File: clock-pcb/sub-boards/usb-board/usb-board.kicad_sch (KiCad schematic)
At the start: 5 parts, among them J1 USB4140-GF-0070-C

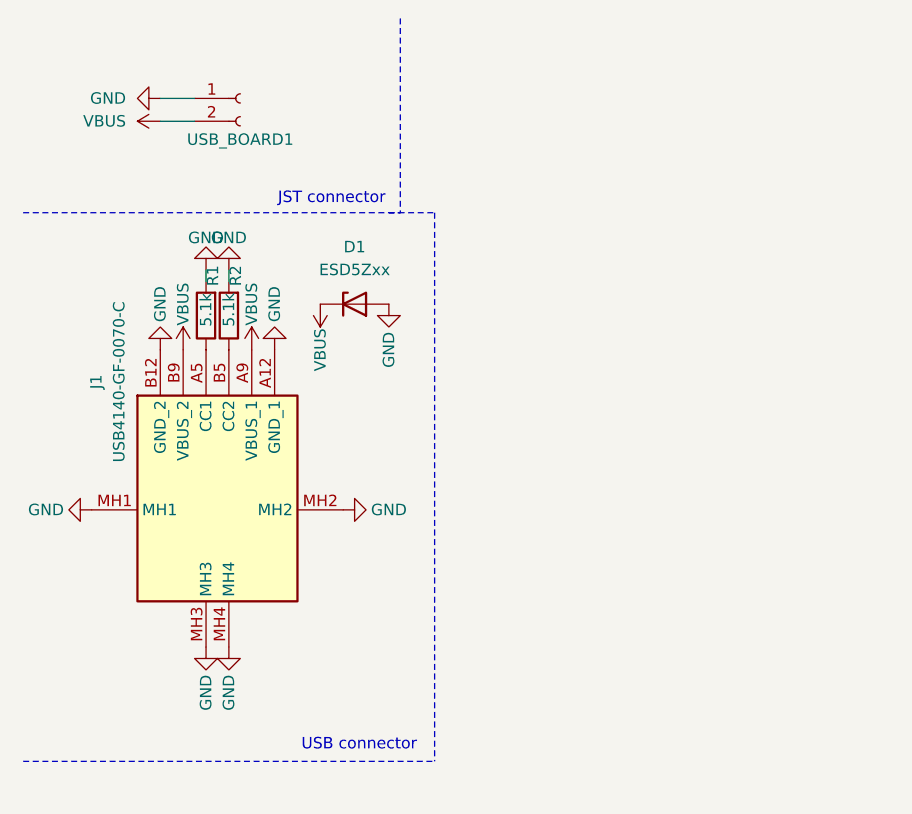
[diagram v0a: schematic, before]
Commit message: new pcb
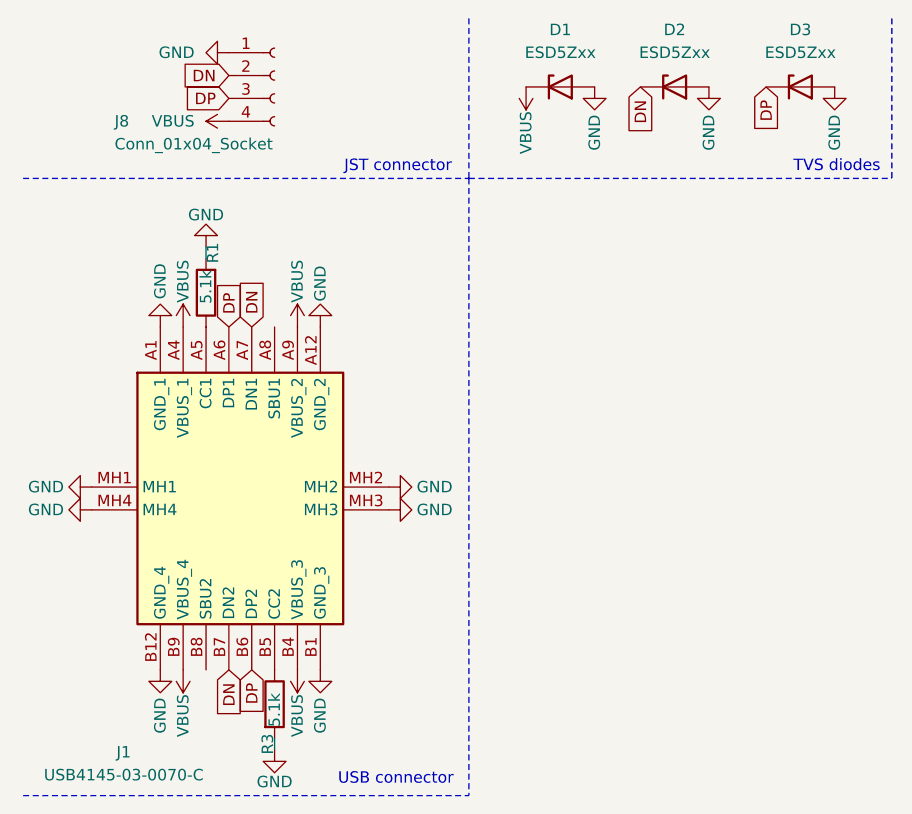
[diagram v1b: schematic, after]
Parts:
- removed J1: USB4140-GF-0070-C, clock:USB4140GF0070C, symbol clock:USB4140-GF-0070-C
- removed R2: 5.1k, Resistor_SMD:R_0402_1005Metric, symbol clock:R
- removed USB_BOARD1: Conn_01x02_Socket, clock:SHDR2W64P0X250_1X2_740X575X700P, symbol clock:Conn_01x02_Socket
- added D2, D3: ESD5Zxx, Diode_SMD:D_SOD-523, symbol clock:ESD5Zxx
- added J1: USB4145-03-0070-C, clock:USB4145030070C, symbol USB4145-03-0070-C:USB4145-03-0070-C
- added J8: Conn_01x04_Socket, Connector_JST:JST_XH_B4B-XH-AM_1x04_P2.50mm_Vertical, symbol Connector:Conn_01x04_Socket
- added R3: 5.1k, Resistor_SMD:R_0402_1005Metric, symbol clock:R
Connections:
- net GND: now also D2.2 (A), D3.2 (A), J1.A1 (GND_1), J1.A12 (GND_2), J1.B1 (GND_3), J1.B12 (GND_4), J1.MH1, J1.MH2, J1.MH3, J1.MH4, J8.1 (Pin_1), R3.2
- net VBUS: now also J1.A4 (VBUS_1), J1.A9 (VBUS_2), J1.B4 (VBUS_3), J1.B9 (VBUS_4), J8.4 (Pin_4)
- net at R1.1: now also J1.A5 (CC1)
- new net: J1.B5 (CC2), R3.1
- new net DN: D2.1 (K), J1.A7 (DN1), J1.B7 (DN2), J8.2 (Pin_2)
- new net DP: D3.1 (K), J1.A6 (DP1), J1.B6 (DP2), J8.3 (Pin_3)
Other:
- note added: "TVS diodes"
- moved on the sheet: D1, R1
